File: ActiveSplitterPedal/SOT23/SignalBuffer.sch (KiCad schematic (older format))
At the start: 4 parts, among them U1 OPA842, U5 DG468DV_T1_E3

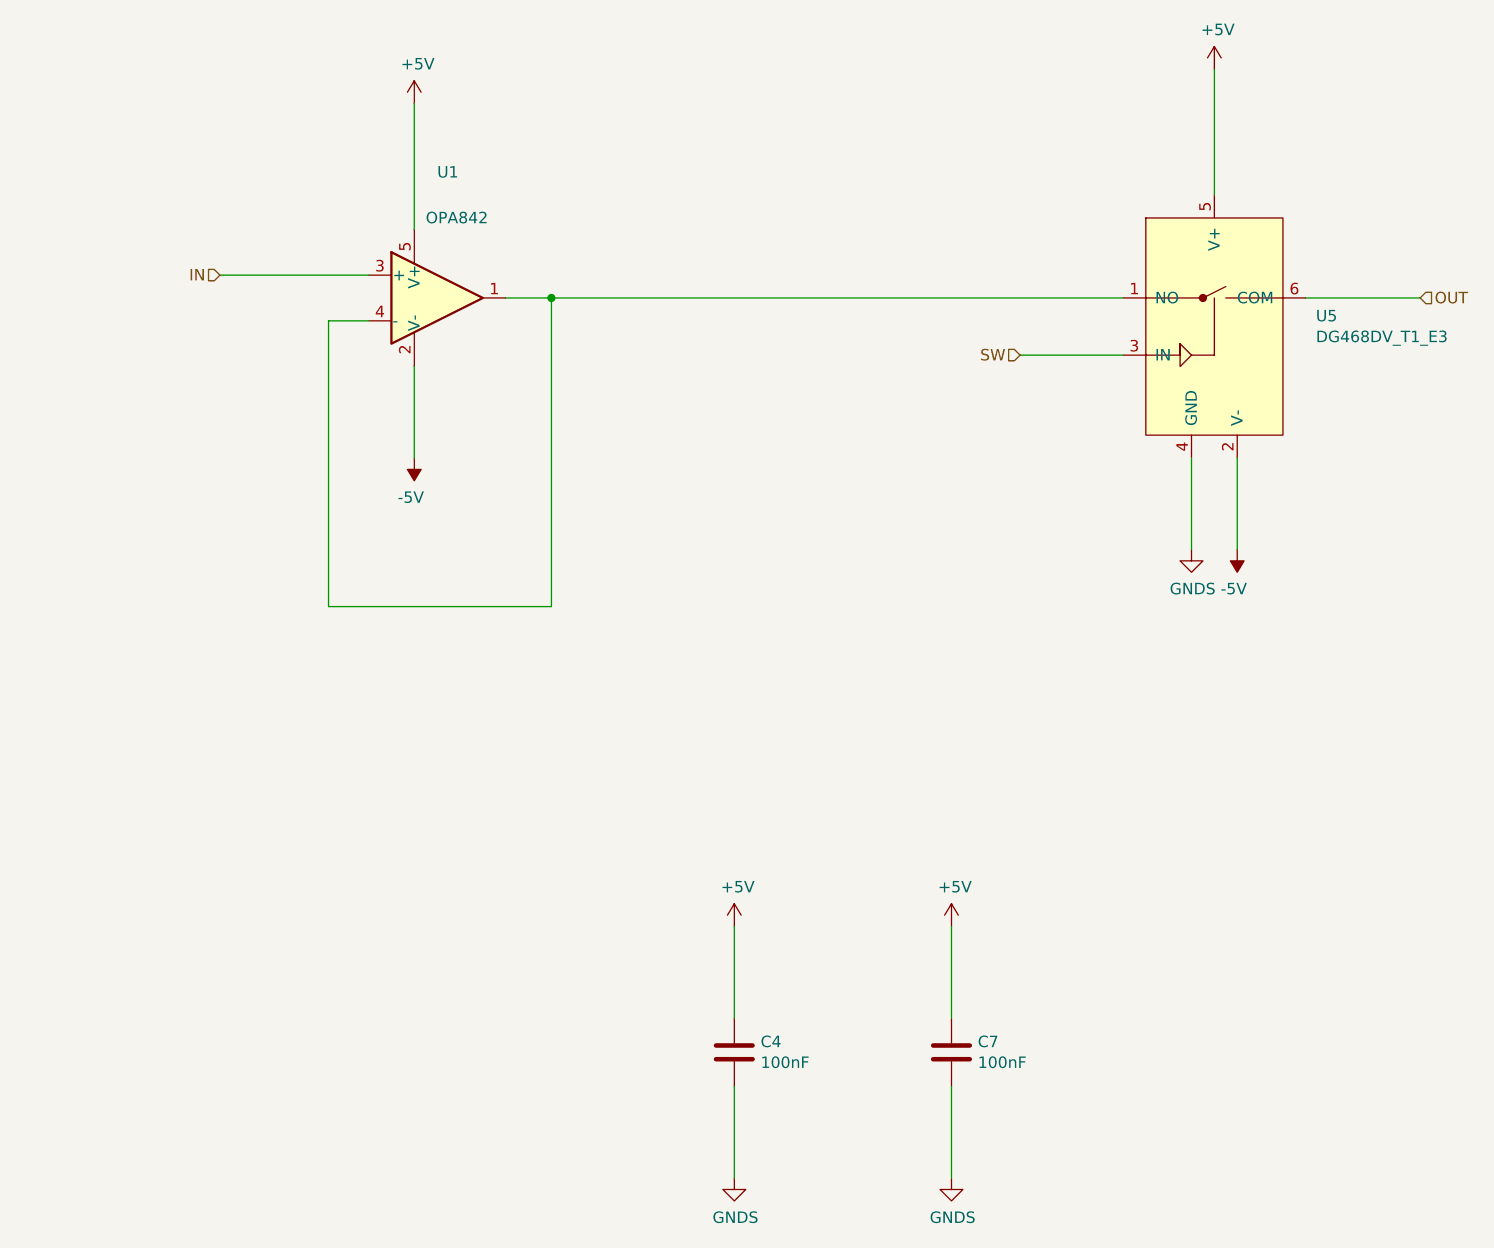
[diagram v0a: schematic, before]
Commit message: updated schematic
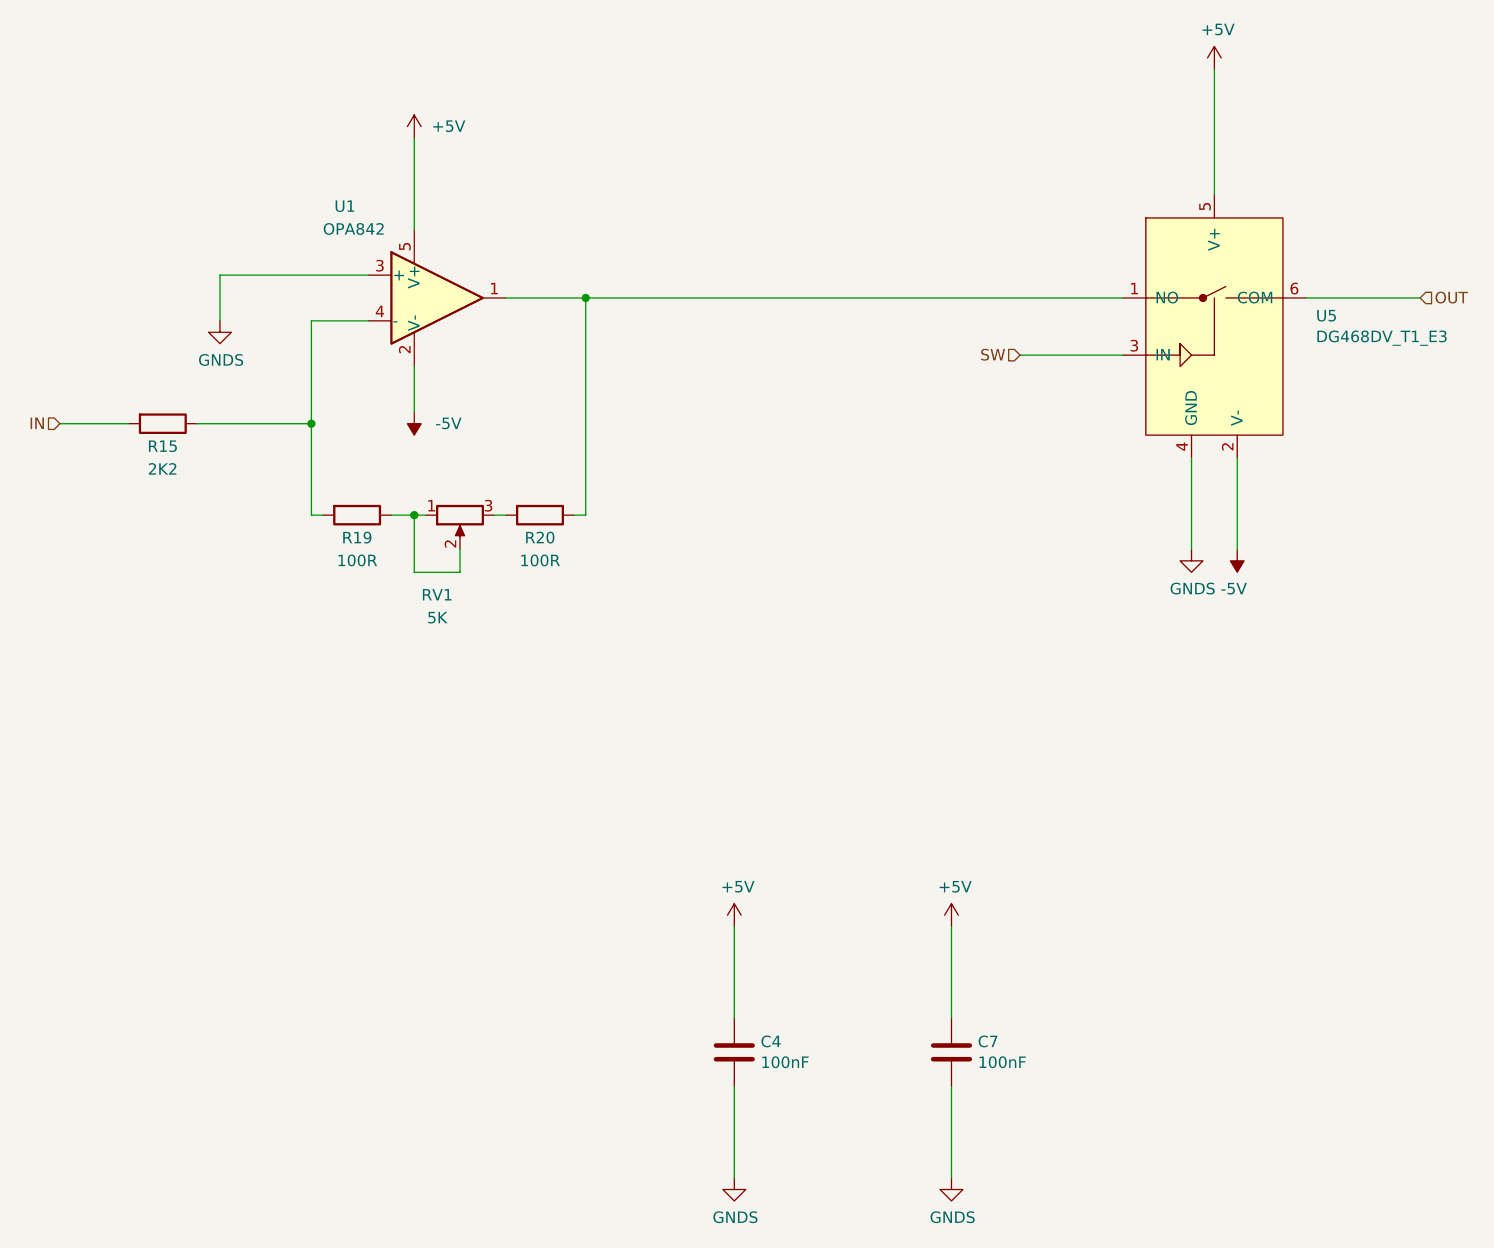
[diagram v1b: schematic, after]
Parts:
- added R15: 2K2, Resistor_SMD:R_0805_2012Metric_Pad1.15x1.40mm_HandSolder, symbol Device:R
- added R19, R20: 100R, Resistor_SMD:R_0805_2012Metric_Pad1.15x1.40mm_HandSolder, symbol Device:R
- added RV1: 5K, Potentiometer_THT:Potentiometer_Alps_RK09L_Single_Vertical, symbol Device:R_POT
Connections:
- net GNDS: now also U1.3 (+)
- net IN: now also R15.2; no longer U1.3 (+)
- net at U1.1, U5.1 (NO): now also R20.1; no longer U1.4 (-)
- new net: R15.1, R19.2, U1.4 (-)
- new net: R19.1, RV1.1, RV1.2
- new net: R20.2, RV1.3
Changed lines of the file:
@@
 $EndDescr
 Wire Wire Line
-	2600 3000 3250 3000
-Wire Wire Line
-	3250 3200 3075 3200
-Wire Wire Line
-	3075 3200 3075 4450
-Wire Wire Line
-	3075 4450 4050 4450
-Wire Wire Line
-	4050 4450 4050 3100
-Wire Wire Line
-	4050 3100 3850 3100
-Wire Wire Line
-	4050 3100 6550 3100
-Connection ~ 4050 3100
+	1900 3650 2200 3650
 Wire Wire Line
 	6550 3350 6100 3350
@@
 Text HLabel 6100 3350 0    50   Input ~ 0
 SW
-Text HLabel 2600 3000 0    50   Input ~ 0
+Text HLabel 1900 3650 0    50   Input ~ 0
 IN
 Text HLabel 7850 3100 2    50   Input ~ 0
 OUT
 $Comp
-L Amplifier_Operational:OPA842xDBV U1
-U 1 1 5F35E576
-P 3550 3100
-AR Path="/5F350192/5F35E576" Ref="U1"  Part="1"
-AR Path="/5F3658F9/5F35E576" Ref="U2"  Part="1"
-AR Path="/5F365961/5F35E576" Ref="U3"  Part="1"
-AR Path="/5F365B82/5F35E576" Ref="U4"  Part="1"
-F 0 "U1" H 3550 3650 50  0000 L CNN
-F 1 "OPA842" H 3500 3450 50  0000 L CNN
-F 2 "Package_TO_SOT_SMD:SOT-23-5" H 3450 2900 50  0001 L CNN
-F 3 "http://www.ti.com/lit/ds/symlink/opa842.pdf" H 3550 3300 50  0001 C CNN
-	1    3550 3100
-	1    0    0    -1
-$EndComp
-Wire Wire Line
-	3450 3400 3450 3800
-$Comp
-L power:-5V #PWR017
-U 1 1 5F361BF5
-P 3450 3800
-AR Path="/5F350192/5F361BF5" Ref="#PWR017"  Part="1"
-AR Path="/5F3658F9/5F361BF5" Ref="#PWR019"  Part="1"
-AR Path="/5F365961/5F361BF5" Ref="#PWR021"  Part="1"
-AR Path="/5F365B82/5F361BF5" Ref="#PWR023"  Part="1"
-F 0 "#PWR017" H 3450 3900 50  0001 C CNN
-F 1 "-5V" H 3465 3973 50  0000 C CNN
-F 2 "" H 3450 3800 50  0001 C CNN
-F 3 "" H 3450 3800 50  0001 C CNN
-	1    3450 3800
-	-1   0    0    1
-$EndComp
-$Comp
 L power:+5V #PWR016
 U 1 1 5F361F40
-P 3450 2250
+P 3450 2400
 AR Path="/5F350192/5F361F40" Ref="#PWR016"  Part="1"
 AR Path="/5F3658F9/5F361F40" Ref="#PWR018"  Part="1"
 AR Path="/5F365961/5F361F40" Ref="#PWR020"  Part="1"
 AR Path="/5F365B82/5F361F40" Ref="#PWR022"  Part="1"
-F 0 "#PWR016" H 3450 2100 50  0001 C CNN
-F 1 "+5V" H 3465 2423 50  0000 C CNN
-F 2 "" H 3450 2250 50  0001 C CNN
-F 3 "" H 3450 2250 50  0001 C CNN
-	1    3450 2250
-	1    0    0    -1
-$EndComp
-Wire Wire Line
-	3450 2250 3450 2800
+F 0 "#PWR016" H 3450 2250 50  0001 C CNN
+F 1 "+5V" H 3600 2450 50  0000 C CNN
+F 2 "" H 3450 2400 50  0001 C CNN
+F 3 "" H 3450 2400 50  0001 C CNN
+	1    3450 2400
+	1    0    0    -1
+$EndComp
+Wire Wire Line
+	3450 2400 3450 2800
 $Comp
 L power:+5V #PWR0101
@@
 	1    0    0    -1
 $EndComp
+$Comp
+L power:-5V #PWR017
+U 1 1 5F361BF5
+P 3450 3600
+AR Path="/5F350192/5F361BF5" Ref="#PWR017"  Part="1"
+AR Path="/5F3658F9/5F361BF5" Ref="#PWR019"  Part="1"
+AR Path="/5F365961/5F361BF5" Ref="#PWR021"  Part="1"
+AR Path="/5F365B82/5F361BF5" Ref="#PWR023"  Part="1"
+F 0 "#PWR017" H 3450 3700 50  0001 C CNN
+F 1 "-5V" H 3300 3650 50  0000 C CNN
+F 2 "" H 3450 3600 50  0001 C CNN
+F 3 "" H 3450 3600 50  0001 C CNN
+	1    3450 3600
+	-1   0    0    1
+$EndComp
+Wire Wire Line
+	3450 3400 3450 3600
+Wire Wire Line
+	4200 3100 6550 3100
+Wire Wire Line
+	4200 3100 3850 3100
+Connection ~ 4200 3100
+Wire Wire Line
+	4200 4050 4200 3100
+Wire Wire Line
+	3000 4050 3050 4050
+Wire Wire Line
+	3000 3200 3000 3650
+Wire Wire Line
+	3250 3200 3000 3200
+$Comp
+L Amplifier_Operational:OPA842xDBV U1
+U 1 1 5F35E576
+P 3550 3100
+AR Path="/5F350192/5F35E576" Ref="U1"  Part="1"
+AR Path="/5F3658F9/5F35E576" Ref="U2"  Part="1"
+AR Path="/5F365961/5F35E576" Ref="U3"  Part="1"
+AR Path="/5F365B82/5F35E576" Ref="U4"  Part="1"
+F 0 "U1" H 3100 3500 50  0000 L CNN
+F 1 "OPA842" H 3050 3400 50  0000 L CNN
+F 2 "Package_TO_SOT_SMD:SOT-23-5" H 3450 2900 50  0001 L CNN
+F 3 "http://www.ti.com/lit/ds/symlink/opa842.pdf" H 3550 3300 50  0001 C CNN
+	1    3550 3100
+	1    0    0    -1
+$EndComp
+$Comp
+L Device:R R15
+U 1 1 5F374B42
+P 2350 3650
+AR Path="/5F350192/5F374B42" Ref="R15"  Part="1"
+AR Path="/5F365B82/5F374B42" Ref="R9"  Part="1"
+AR Path="/5F365961/5F374B42" Ref="R11"  Part="1"
+AR Path="/5F3658F9/5F374B42" Ref="R13"  Part="1"
+F 0 "R15" V 2450 3650 50  0000 C CNN
+F 1 "2K2" V 2550 3650 50  0000 C CNN
+F 2 "Resistor_SMD:R_0805_2012Metric_Pad1.15x1.40mm_HandSolder" V 2280 3650 50  0001 C CNN
+F 3 "~" H 2350 3650 50  0001 C CNN
+	1    2350 3650
+	0    1    1    0
+$EndComp
+Wire Wire Line
+	2500 3650 3000 3650
+Wire Wire Line
+	3800 4050 3850 4050
+Connection ~ 3000 3650
+Wire Wire Line
+	3000 3650 3000 4050
+Wire Wire Line
+	3250 3000 2600 3000
+Wire Wire Line
+	2600 3000 2600 3200
+$Comp
+L power:GNDS #PWR047
+U 1 1 5F377EED
+P 2600 3200
+AR Path="/5F350192/5F377EED" Ref="#PWR047"  Part="1"
+AR Path="/5F365B82/5F377EED" Ref="#PWR044"  Part="1"
+AR Path="/5F365961/5F377EED" Ref="#PWR045"  Part="1"
+AR Path="/5F3658F9/5F377EED" Ref="#PWR046"  Part="1"
+F 0 "#PWR047" H 2600 2950 50  0001 C CNN
+F 1 "GNDS" H 2605 3027 50  0000 C CNN
+F 2 "" H 2600 3200 50  0001 C CNN
+F 3 "" H 2600 3200 50  0001 C CNN
+	1    2600 3200
+	1    0    0    -1
+$EndComp
+$Comp
+L Device:R_POT RV1
+U 1 1 5F37ADE4
+P 3650 4050
+AR Path="/5F350192/5F37ADE4" Ref="RV1"  Part="1"
+AR Path="/5F365B82/5F37ADE4" Ref="RV4"  Part="1"
+AR Path="/5F365961/5F37ADE4" Ref="RV3"  Part="1"
+AR Path="/5F3658F9/5F37ADE4" Ref="RV2"  Part="1"
+F 0 "RV1" V 4000 4150 50  0000 C CNN
+F 1 "5K" V 4100 4150 50  0000 C CNN
+F 2 "Potentiometer_THT:Potentiometer_Alps_RK09L_Single_Vertical" H 3650 4050 50  0001 C CNN
+F 3 "https://docs.rs-online.com/3ea0/0900766b80f4c570.pdf" H 3650 4050 50  0001 C CNN
+	1    3650 4050
+	0    -1   1    0
+$EndComp
+Wire Wire Line
+	3650 4200 3650 4300
+Wire Wire Line
+	3650 4300 3450 4300
+Wire Wire Line
+	3450 4300 3450 4050
+Connection ~ 3450 4050
+Wire Wire Line
+	3450 4050 3500 4050
+$Comp
+L Device:R R19
+U 1 1 5F37F653
+P 3200 4050
+AR Path="/5F350192/5F37F653" Ref="R19"  Part="1"
+AR Path="/5F365B82/5F37F653" Ref="R10"  Part="1"
+AR Path="/5F365961/5F37F653" Ref="R14"  Part="1"
+AR Path="/5F3658F9/5F37F653" Ref="R17"  Part="1"
+F 0 "R19" V 3300 4050 50  0000 C CNN
+F 1 "100R" V 3400 4050 50  0000 C CNN
+F 2 "Resistor_SMD:R_0805_2012Metric_Pad1.15x1.40mm_HandSolder" V 3130 4050 50  0001 C CNN
+F 3 "~" H 3200 4050 50  0001 C CNN
+	1    3200 4050
+	0    1    1    0
+$EndComp
+Wire Wire Line
+	3350 4050 3450 4050
+$Comp
+L Device:R R20
+U 1 1 5F37FC84
+P 4000 4050
+AR Path="/5F350192/5F37FC84" Ref="R20"  Part="1"
+AR Path="/5F365B82/5F37FC84" Ref="R12"  Part="1"
+AR Path="/5F365961/5F37FC84" Ref="R16"  Part="1"
+AR Path="/5F3658F9/5F37FC84" Ref="R18"  Part="1"
+F 0 "R20" V 4100 4050 50  0000 C CNN
+F 1 "100R" V 4200 4050 50  0000 C CNN
+F 2 "Resistor_SMD:R_0805_2012Metric_Pad1.15x1.40mm_HandSolder" V 3930 4050 50  0001 C CNN
+F 3 "~" H 4000 4050 50  0001 C CNN
+	1    4000 4050
+	0    1    1    0
+$EndComp
+Wire Wire Line
+	4150 4050 4200 4050
 $EndSCHEMATC
